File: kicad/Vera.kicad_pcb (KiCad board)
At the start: 4 copper layers, 46 x 48 mm, 37 parts, among them Q1 AO3400, T1 Wurth 749010012A, T2 Wurth 749010012A, U1 TI AM62A7, U2 Microchip KSZ9477, U3 TI MSPM0G3507, U4 TI ISOW1044BDFMR, U5 Infineon SLB9670, Y1 25MHz

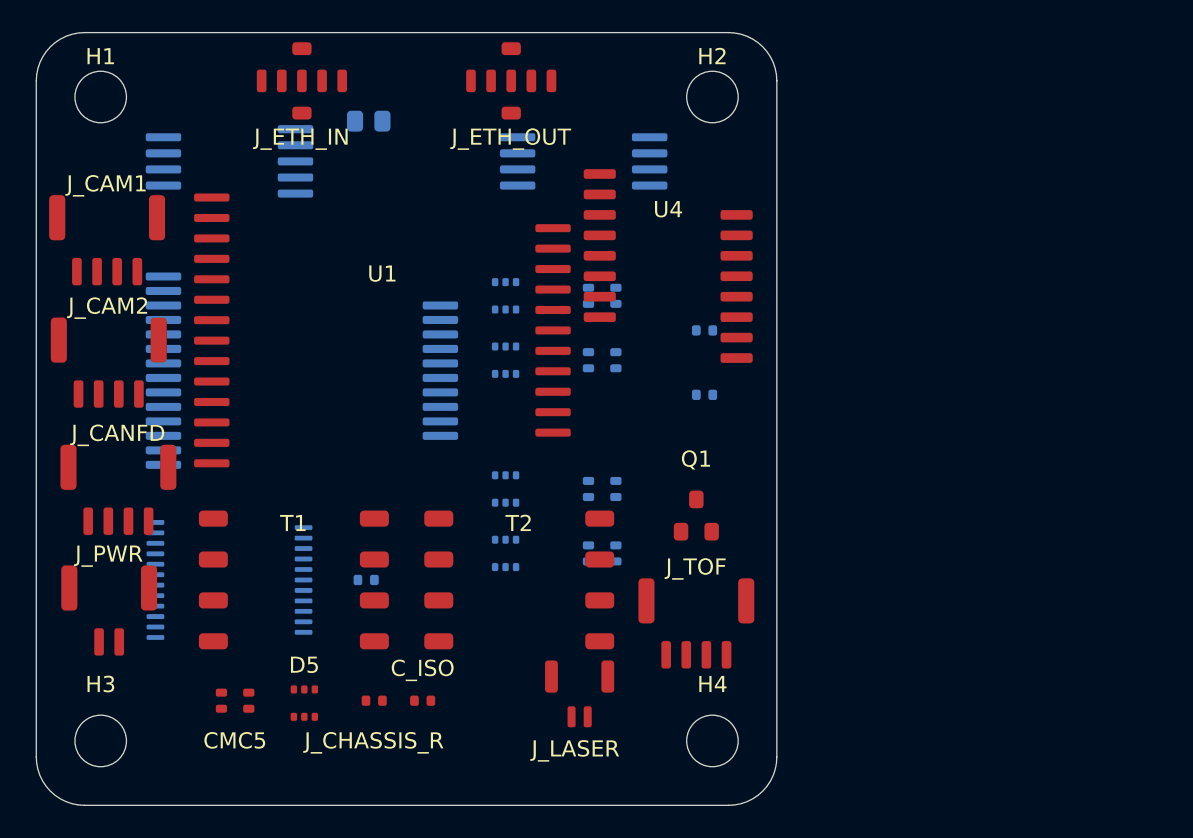
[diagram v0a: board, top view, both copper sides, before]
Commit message: updates to airframe and manual updates to vera.
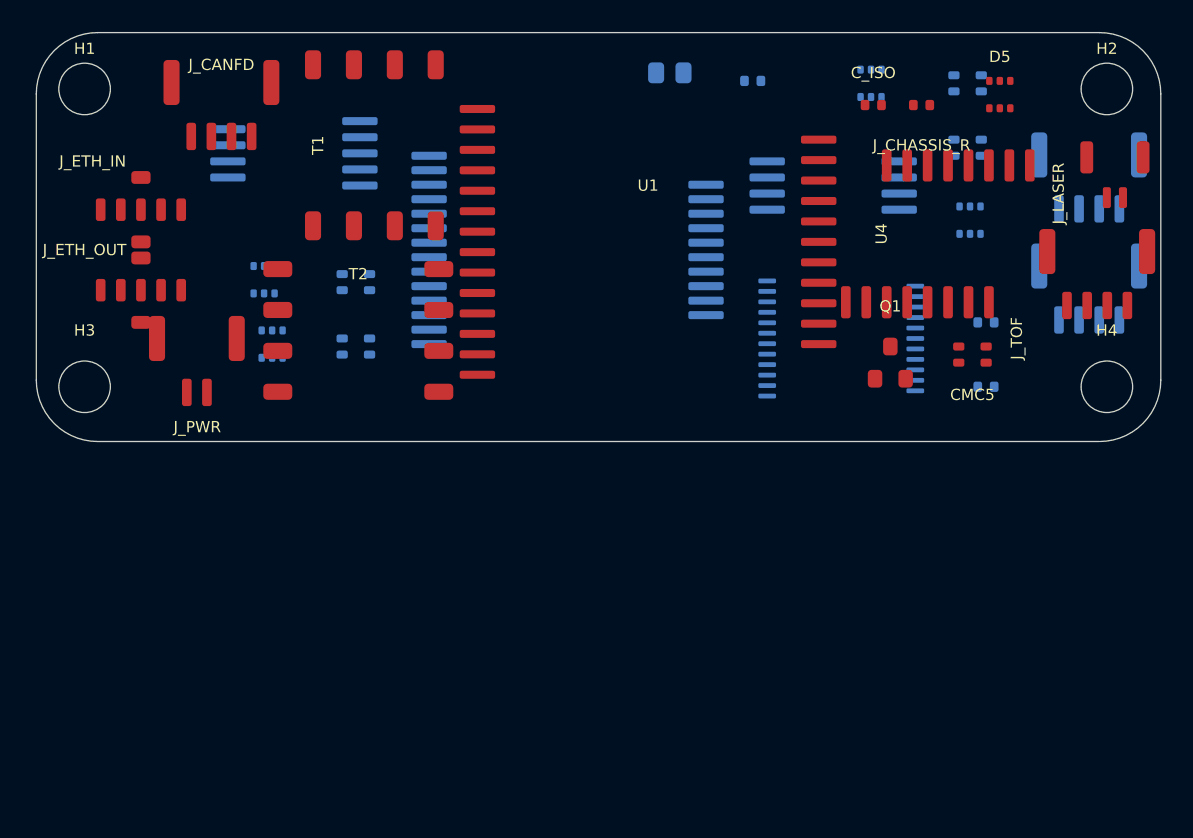
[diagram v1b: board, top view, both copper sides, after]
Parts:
- J_CAM1, J_CAM2: moved to B.Cu
- moved J_CAM2 62.0 mm to (65.4, 9.00), turned to 180 degrees
- moved J_CAM1 61.1 mm to (65.4, 15.9), turned to 180 degrees
- moved D5 57.4 mm to (59.9, 3.85)
- moved CMC5 50.6 mm to (58.1, 20.0)
- moved J_CHASSIS_R 50.2 mm to (55.0, 4.50)
- moved C_ISO 46.4 mm to (52.0, 4.50)
- moved J_LASER 46.3 mm to (67.0, 8.75)
- moved U3 40.9 mm to (50.0, 19.0)
- moved C_MCU1 39.2 mm to (44.5, 3.00)
- moved J_TOF 33.0 mm to (65.9, 15.0)
- moved H4 32.9 mm to (66.5, 22.0)
- moved D2 30.1 mm to (58.0, 11.7)
- moved T1 27.5 mm to (21.0, 7.00), turned to 90 degrees
- moved J_ETH_OUT 26.4 mm to (6.50, 16.0)
- moved CMC1 26.3 mm to (57.9, 3.15)
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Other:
- board size 46 x 48 mm -> 69.8 x 25.4 mm
- copper layers 4 -> 3
